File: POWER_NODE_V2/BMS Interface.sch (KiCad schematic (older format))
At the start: 0 parts

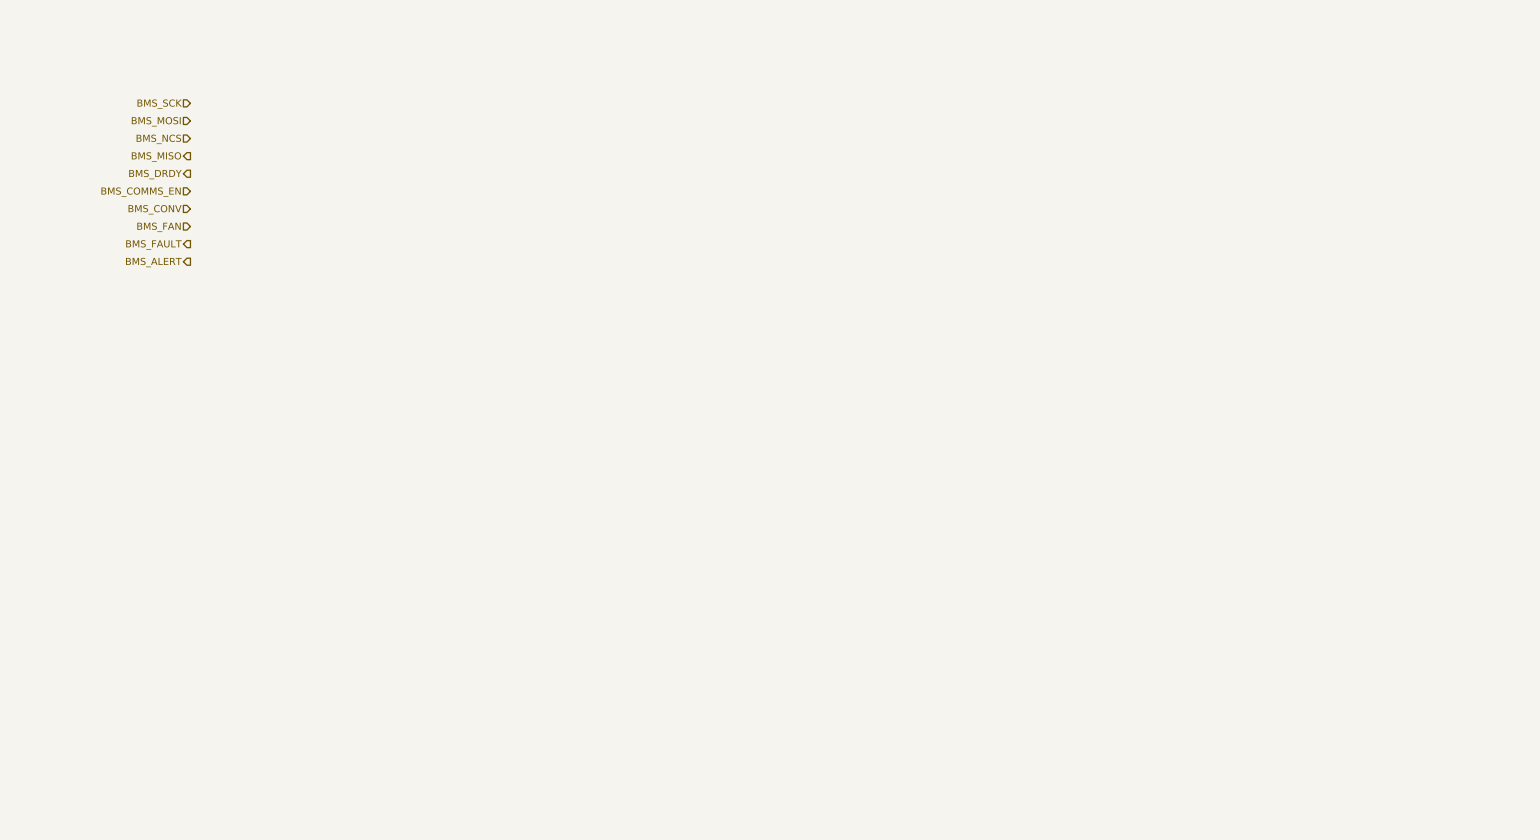
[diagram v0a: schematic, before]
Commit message: WIP
making good progress
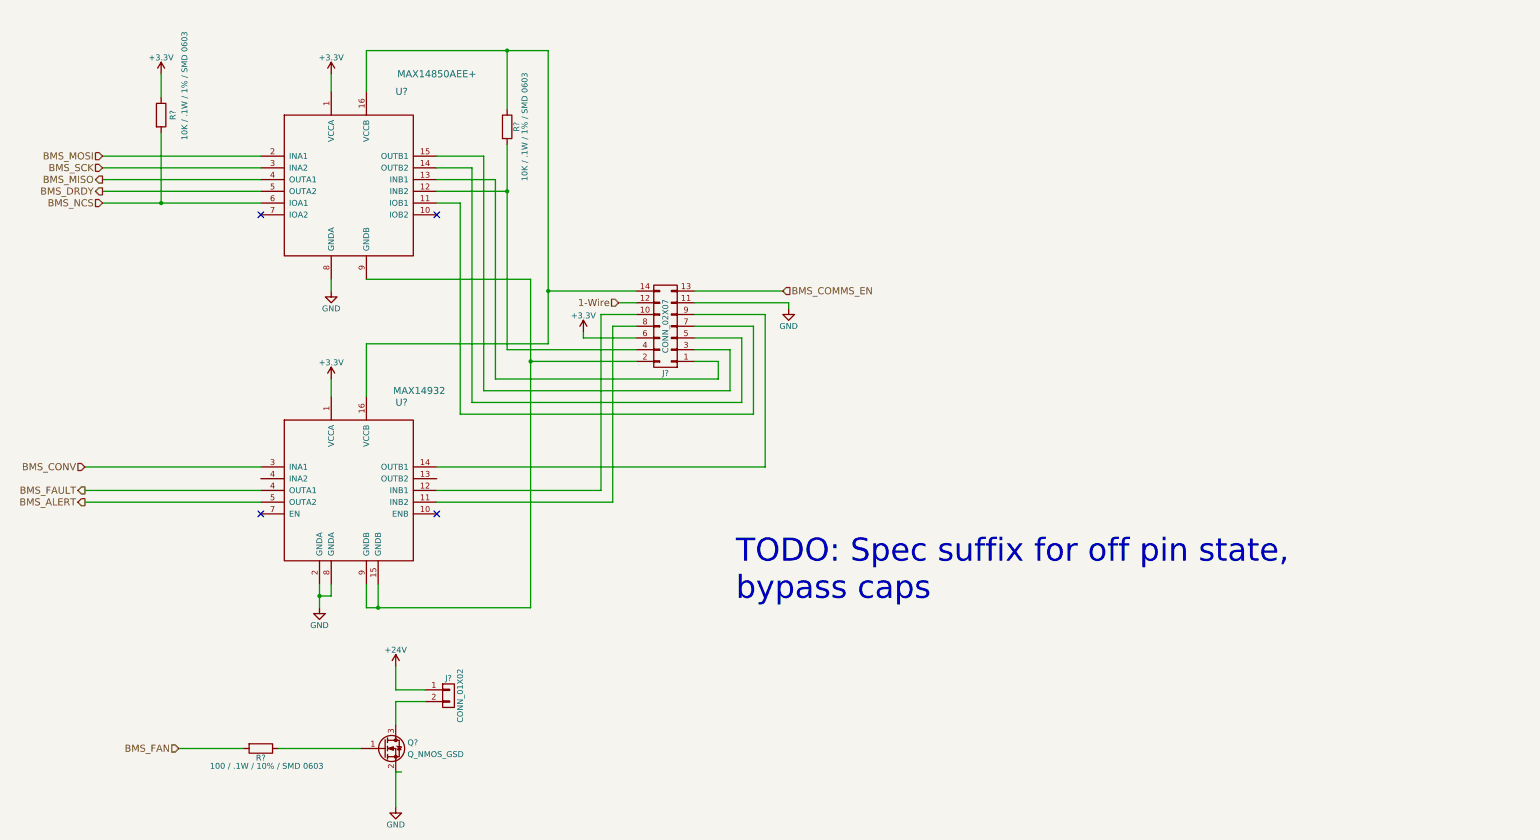
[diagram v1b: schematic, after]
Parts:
- added J?: CONN_02X07, symbol CONN_02X07
- added J?: CONN_01X02, symbol CONN_01X02
- added Q?: Q_NMOS_GSD, symbol Q_NMOS_GSD
- added R? (x2): 10K / .1W / 1% / SMD 0603, symbol R
- added R?: 100 / .1W / 10% / SMD 0603, symbol R
- added U?: MAX14850AEE+, symbol MAX14850AEE+
- added U?: MAX14932, symbol MAX14932
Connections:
- net BMS_ALERT: now also U?.5 (OUTA2)
- net BMS_COMMS_EN: now also J?.13 (P13)
- net BMS_CONV: now also U?.3 (INA1)
- net BMS_DRDY: now also U?.5 (OUTA2)
- net BMS_FAN: now also R?.2
- net BMS_FAULT: now also U?.4 (OUTA1)
- net BMS_MISO: now also U?.4 (OUTA1)
- net BMS_MOSI: now also U?.2 (INA1)
- net BMS_NCS: now also R?.2, U?.6 (IOA1)
- net BMS_SCK: now also U?.3 (INA2)
- new net: J?.7 (P7), U?.11 (IOB1)
- new net: J?.4 (P4), R?.2, U?.12 (INB2)
- new net: J?.1 (P1), U?.13 (INB1)
- new net: J?.5 (P5), U?.14 (OUTB2)
- new net: J?.3 (P3), U?.15 (OUTB1)
- new net: J?.14 (P14), R?.1, U?.16 (VCCB), U?.16 (VCCB)
- new net: J?.2 (P2), U?.15 (GNDB), U?.9 (GNDB), U?.9 (GNDB)
- new net: J?.8 (P8), U?.11 (INB2)
- new net: J?.10 (P10), U?.12 (INB1)
- new net: J?.9 (P9), U?.14 (OUTB1)
- new net: J?.2 (P2), Q?.3 (D)
- new net: Q?.1 (G), R?.1
- new net +24V: J?.1 (P1)
- new net +3V3: J?.6 (P6), R?.1, U?.1 (VCCA), U?.1 (VCCA)
- new net 1-Wire: J?.12 (P12)
- new net GND: J?.11 (P11), Q?.2 (S), U?.2 (GNDA), U?.8 (GNDA), U?.8 (GNDA)
- no-connect marks 0 -> 4
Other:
- note added: "TODO: Spec suffix for off pin state,\nbypass caps\n"
